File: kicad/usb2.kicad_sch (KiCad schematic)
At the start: 10 parts, among them U17 74LVC1G07SE-7

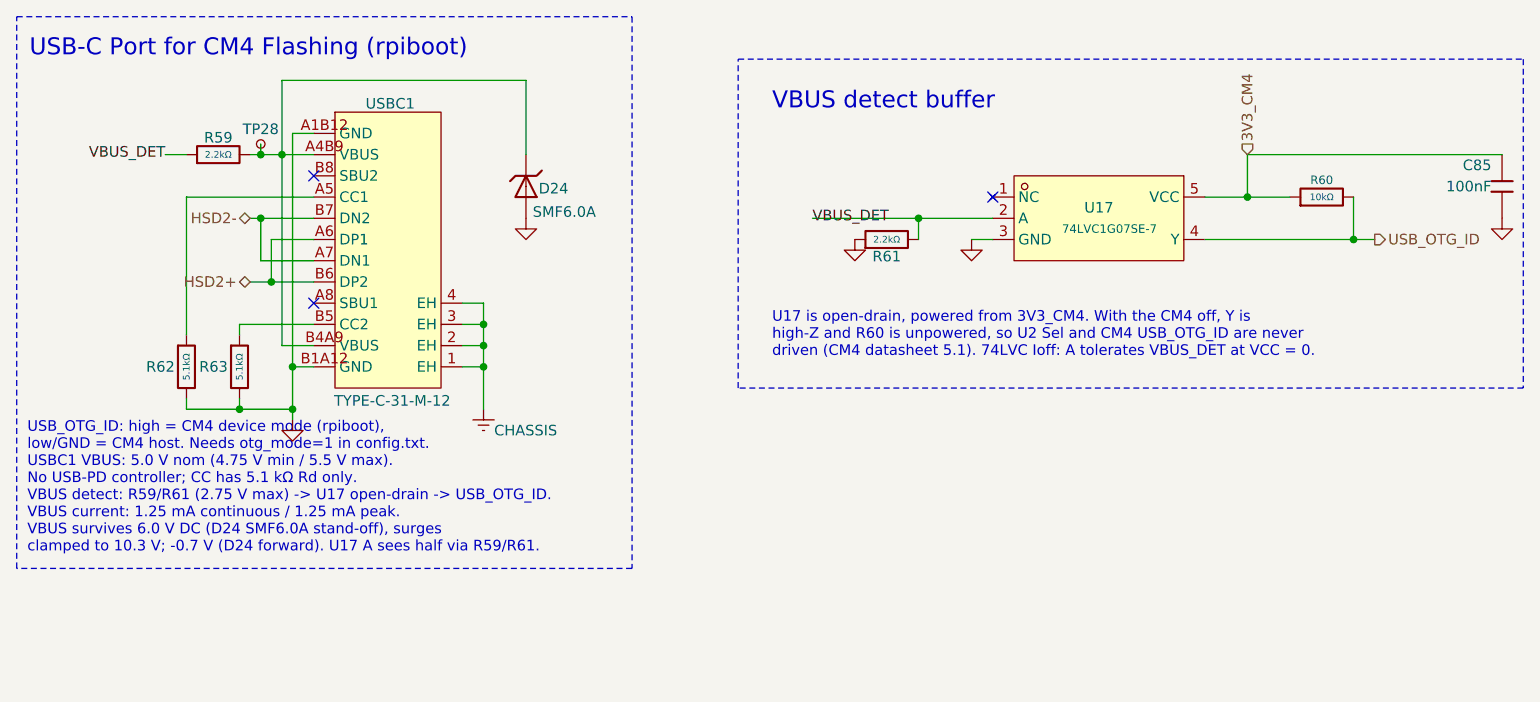
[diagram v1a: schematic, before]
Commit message: Added notes
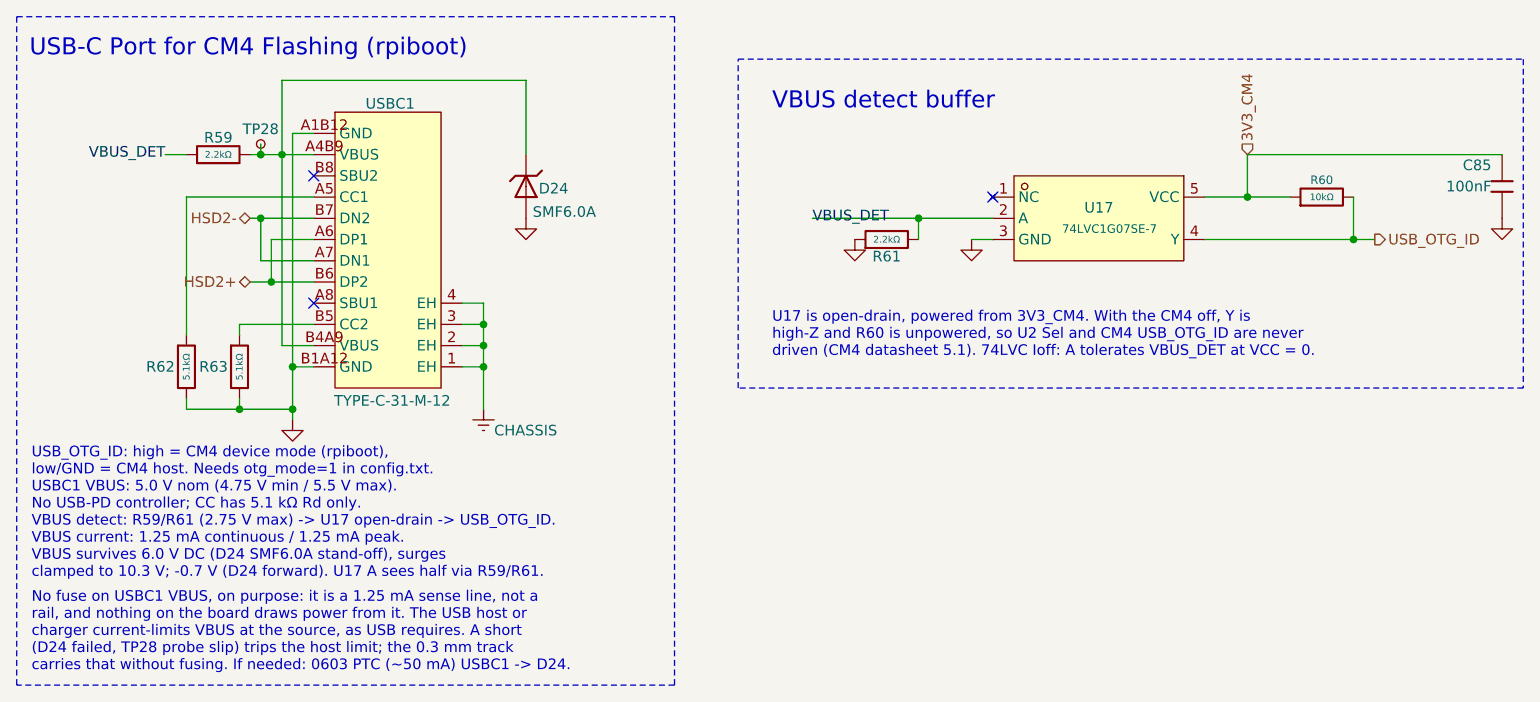
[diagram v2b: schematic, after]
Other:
- note added: "No fuse on USBC1 VBUS, on purpose: it is a 1.25 mA sense line, not a rail, and nothing on the board draws power from it. The USB host or charger current-limits VBUS at the source, as USB requires. A short (D24 failed, TP28 probe slip) trips the host limit; the 0.3 mm track carries that without fusing. If needed: 0603 PTC (~50 mA) USBC1 -> D24."
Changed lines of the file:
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@@
 	(rectangle
 		(start 25.4 25.4)
-		(end 99.06 91.44)
+		(end 104.14 105.41)
 		(stroke
 			(width 0)
@@
 		)
 	)
+	(text "No fuse on USBC1 VBUS, on purpose: it is a 1.25 mA sense line, not a\nrail, and nothing on the board draws power from it. The USB host or\ncharger current-limits VBUS at the source, as USB requires. A short\n(D24 failed, TP28 probe slip) trips the host limit; the 0.3 mm track\ncarries that without fusing. If needed: 0603 PTC (~50 mA) USBC1 -> D24."
+		(exclude_from_sim no)
+		(at 27.178 94.234 0)
+		(effects
+			(font
+				(size 1.27 1.27)
+			)
+			(justify left top)
+		)
+	)
 	(text "USB_OTG_ID: high = CM4 device mode (rpiboot), \nlow/GND = CM4 host. Needs otg_mode=1 in config.txt.\nUSBC1 VBUS: 5.0 V nom (4.75 V min / 5.5 V max).\nNo USB-PD controller; CC has 5.1 kΩ Rd only.\nVBUS detect: R59/R61 (2.75 V max) -> U17 open-drain -> USB_OTG_ID.\nVBUS current: 1.25 mA continuous / 1.25 mA peak.\nVBUS survives 6.0 V DC (D24 SMF6.0A stand-off), surges\nclamped to 10.3 V; -0.7 V (D24 forward). U17 A sees half via R59/R61."
 		(exclude_from_sim no)
-		(at 26.67 81.788 0)
+		(at 27.178 84.836 0)
 		(effects
 			(font
